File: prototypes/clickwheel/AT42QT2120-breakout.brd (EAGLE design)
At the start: 52.1 x 31.4 mm, 5 parts

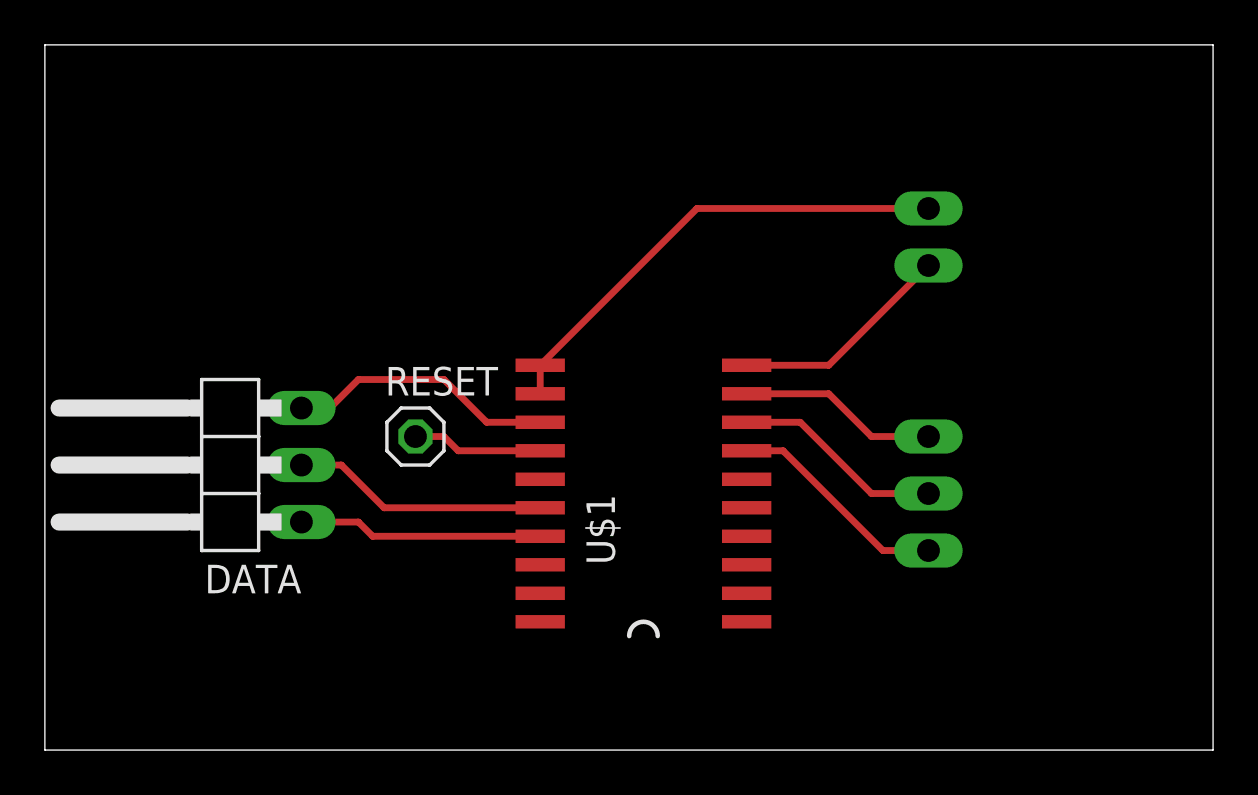
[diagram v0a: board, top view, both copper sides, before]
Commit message: a wheel prototype!
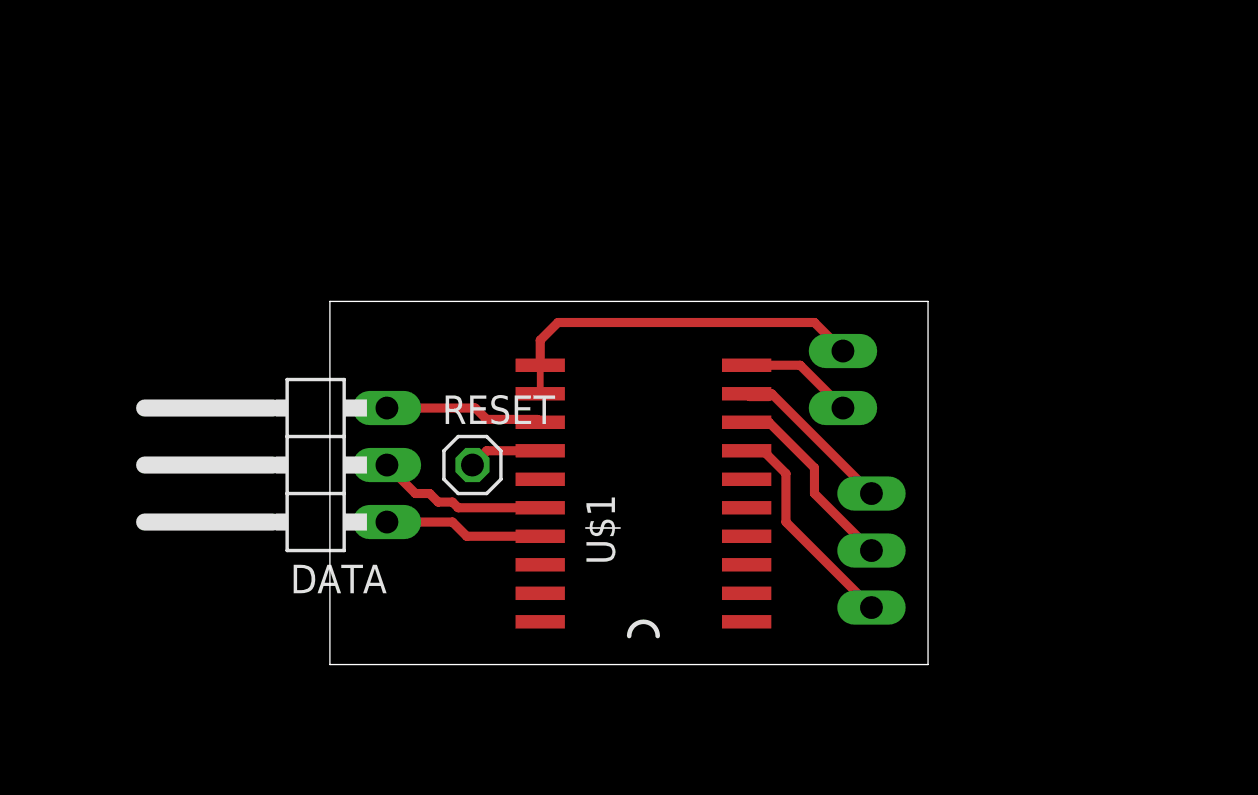
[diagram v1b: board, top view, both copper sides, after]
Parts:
- moved POWER 7.41 mm to (47.0, 25.4)
- moved DATA 3.81 mm to (19.1, 21.6)
- moved CLICKWHEEL 3.59 mm to (48.3, 17.8)
- moved RESET 2.84 mm to (26.7, 21.6)
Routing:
- net N$8: track 12.0 -> 7.09 mm
- net GND: track 21.5 -> 16.7 mm
- net N$4: track 11.4 -> 7.62 mm
- net N$2: track 10.9 -> 7.09 mm
- net V3P3: track 9.94 -> 6.19 mm
- net N$1: track 5.82 -> 3.28 mm
- net N$6: track 9.42 -> 8.60 mm
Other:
- board size 52.1 x 31.4 mm -> 26.6 x 16.2 mm
